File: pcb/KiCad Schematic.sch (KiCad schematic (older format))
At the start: 88 parts, among them IC1 MC7805BDTRKG, IC2 ATSAMD51J19A-MU, J1 47309-3351, J10 Conn_01x04, J11 Conn_01x04, J12 Conn_01x03, J13 Conn_01x03, J14 Conn_01x20, J15 Conn_01x03, J16 Conn_01x03, J17 Hole, J18 Hole, J19 Hole, J2 Conn_01x02, J20 Hole, J21 Conn_01x02, J3 47346-0001, J4 Conn_01x04, J5 Conn_01x04, J6 20021121-00010C4LF, J7 Conn_01x02, J8 Conn_01x02, J9 Conn_01x02, Q1 NVTFS5C680NLTAG, Q2 NVTFS5C680NLTAG, U1 TMC2041-LA, U2 TMC2041-LA, U3 AP2112K-3.3, Y1 LFXTAL009678REEL

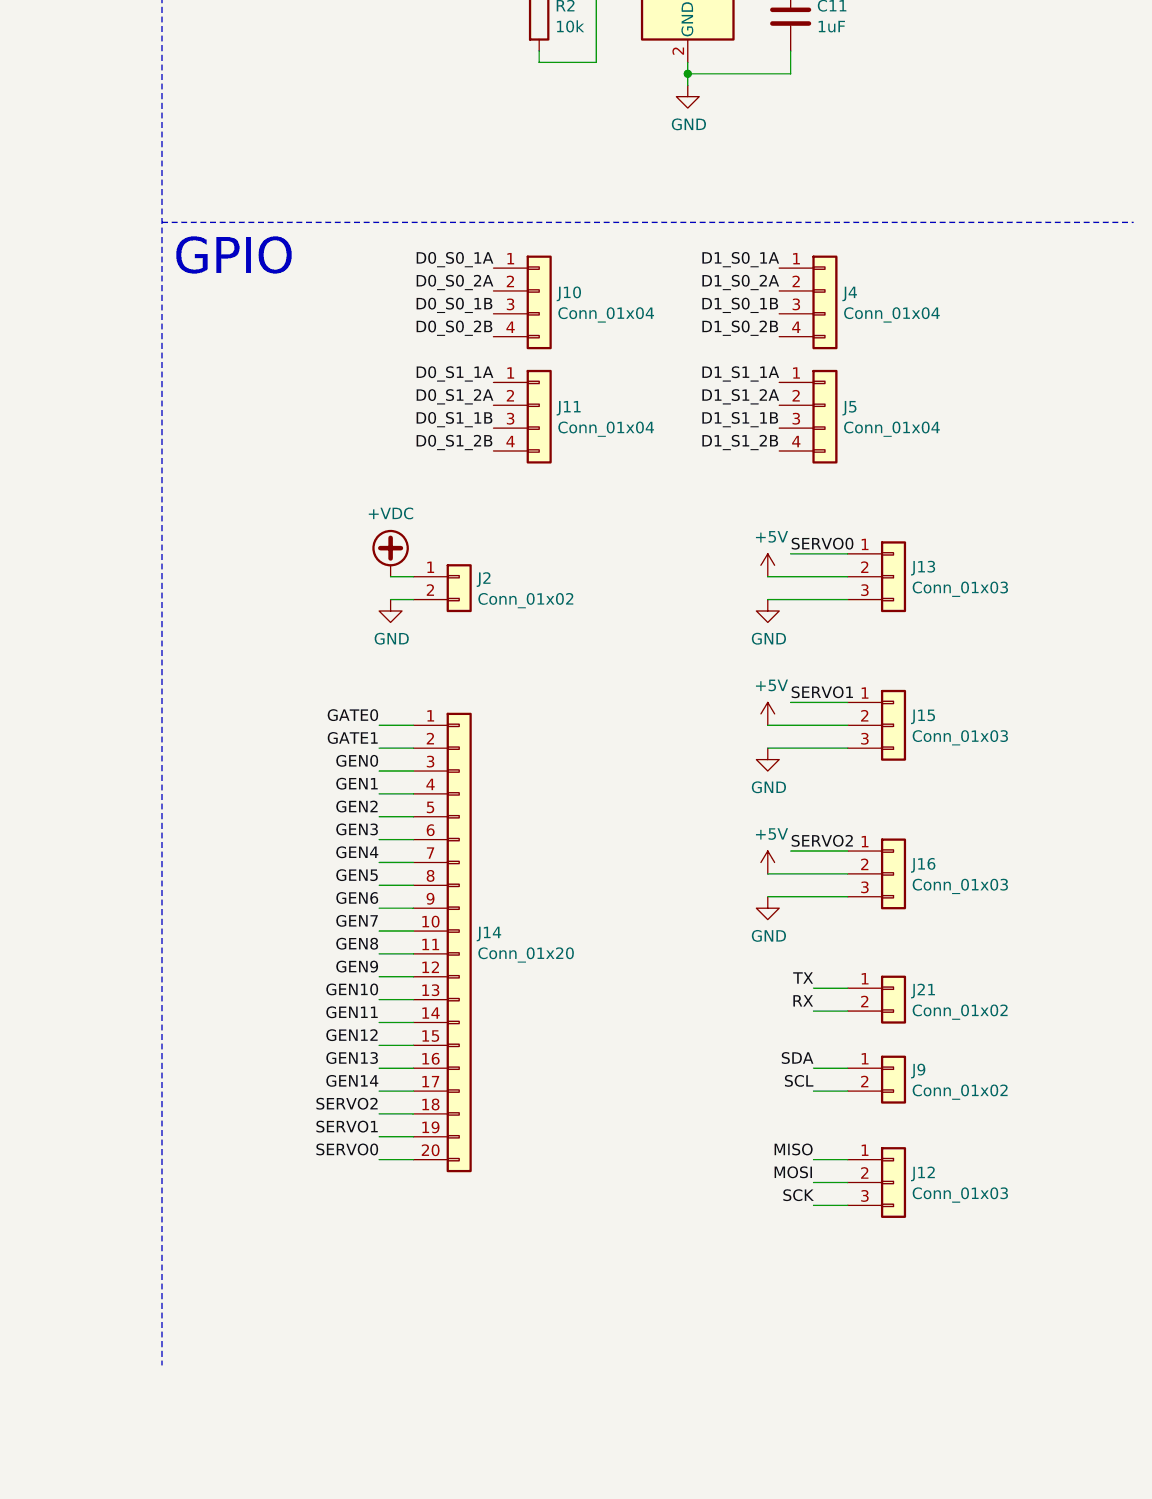
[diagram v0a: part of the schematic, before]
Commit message: add power header
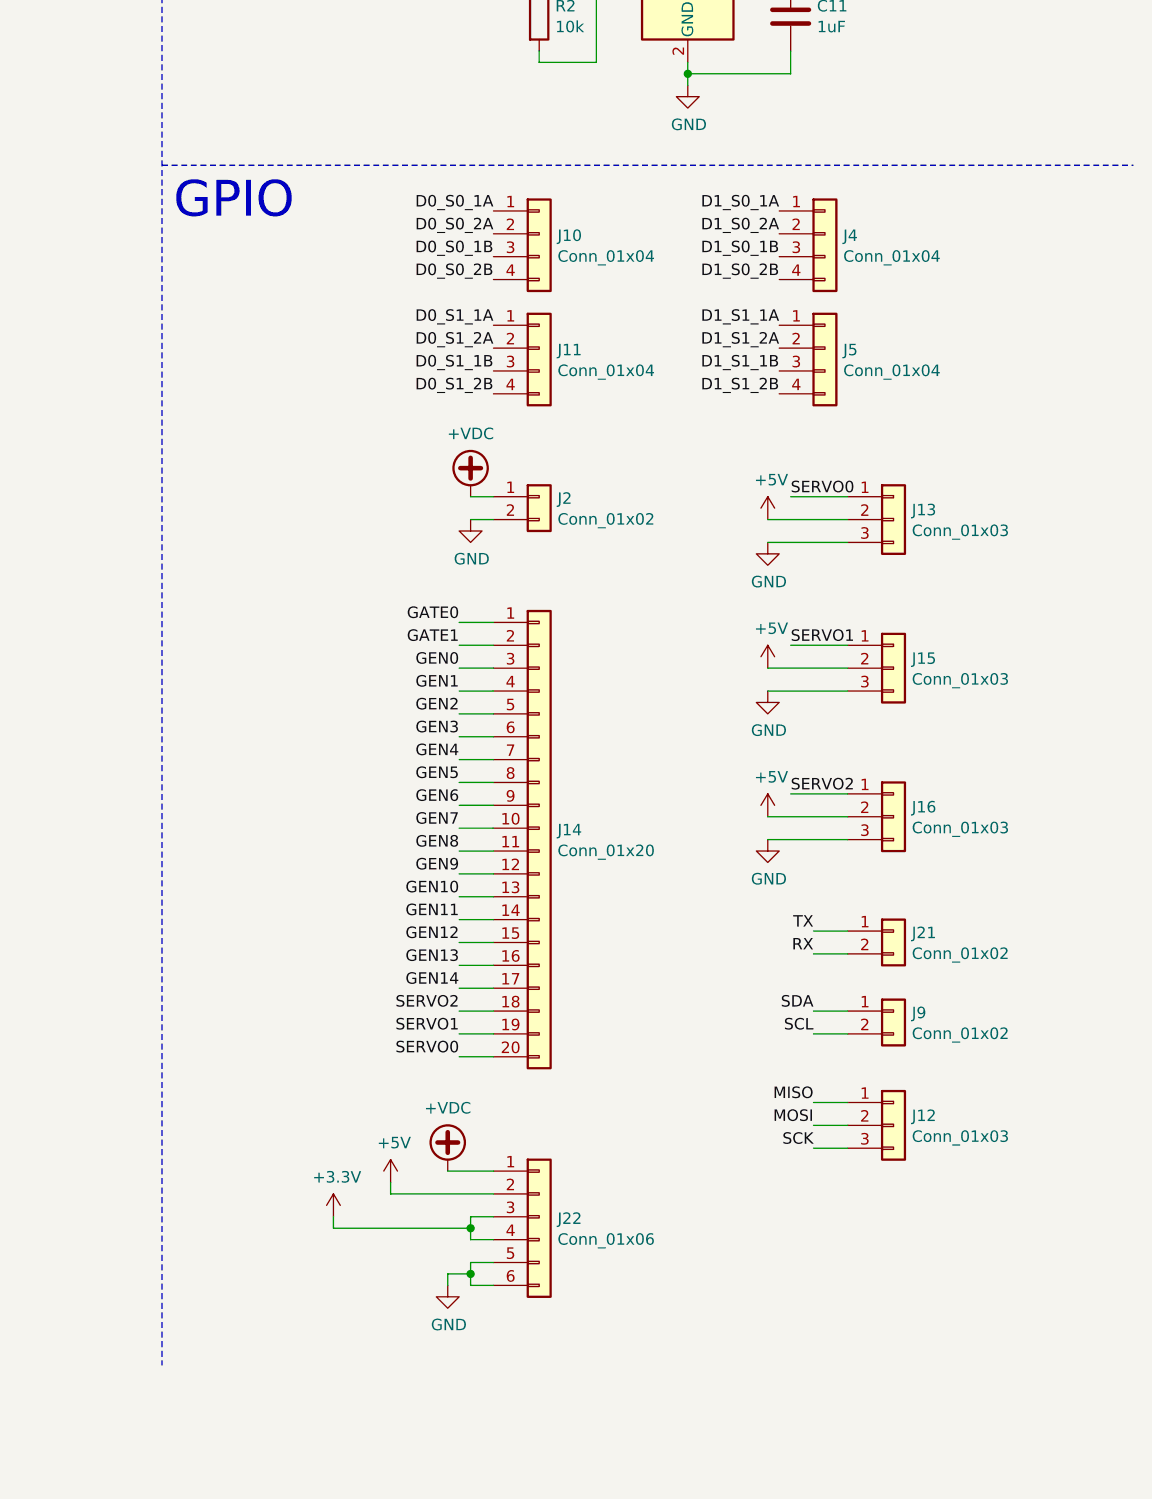
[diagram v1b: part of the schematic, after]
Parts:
- added J22: Conn_01x06, Connector_PinSocket_2.54mm:PinSocket_1x06_P2.54mm_Vertical, symbol Connector_Generic:Conn_01x06
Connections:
- net +3V3: now also J22.3 (Pin_3), J22.4 (Pin_4)
- net +5V: now also J22.2 (Pin_2)
- net +VDC: now also J22.1 (Pin_1)
- net GND: now also J22.5 (Pin_5), J22.6 (Pin_6)
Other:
- moved on the sheet: J10, J11, J12, J13, J14, J15, J16, J2, J21, J4, J5, J9
